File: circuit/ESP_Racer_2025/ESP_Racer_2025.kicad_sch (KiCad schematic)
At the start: 20 parts, among them IC1 XCL102D333CR-G, J1 Conn_LED_1, J2 Conn_LED_2, J3 Conn_Servo, U1 DRV8835DSST, U2 SFV12R-2STE1LF, U3 ESP32-C3-WROOM-02

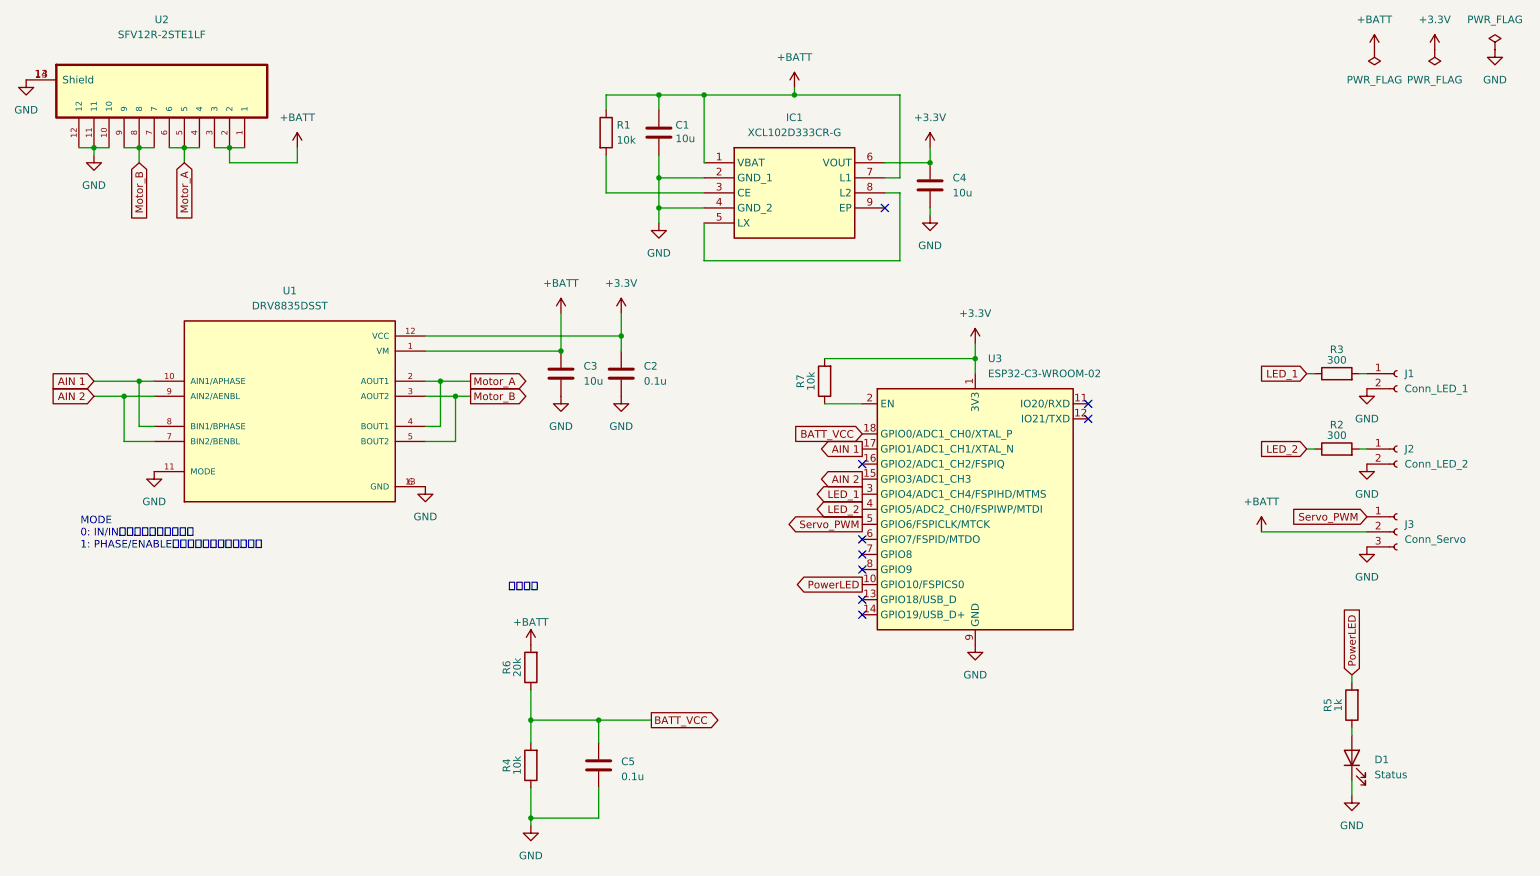
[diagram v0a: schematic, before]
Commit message: fix pcb
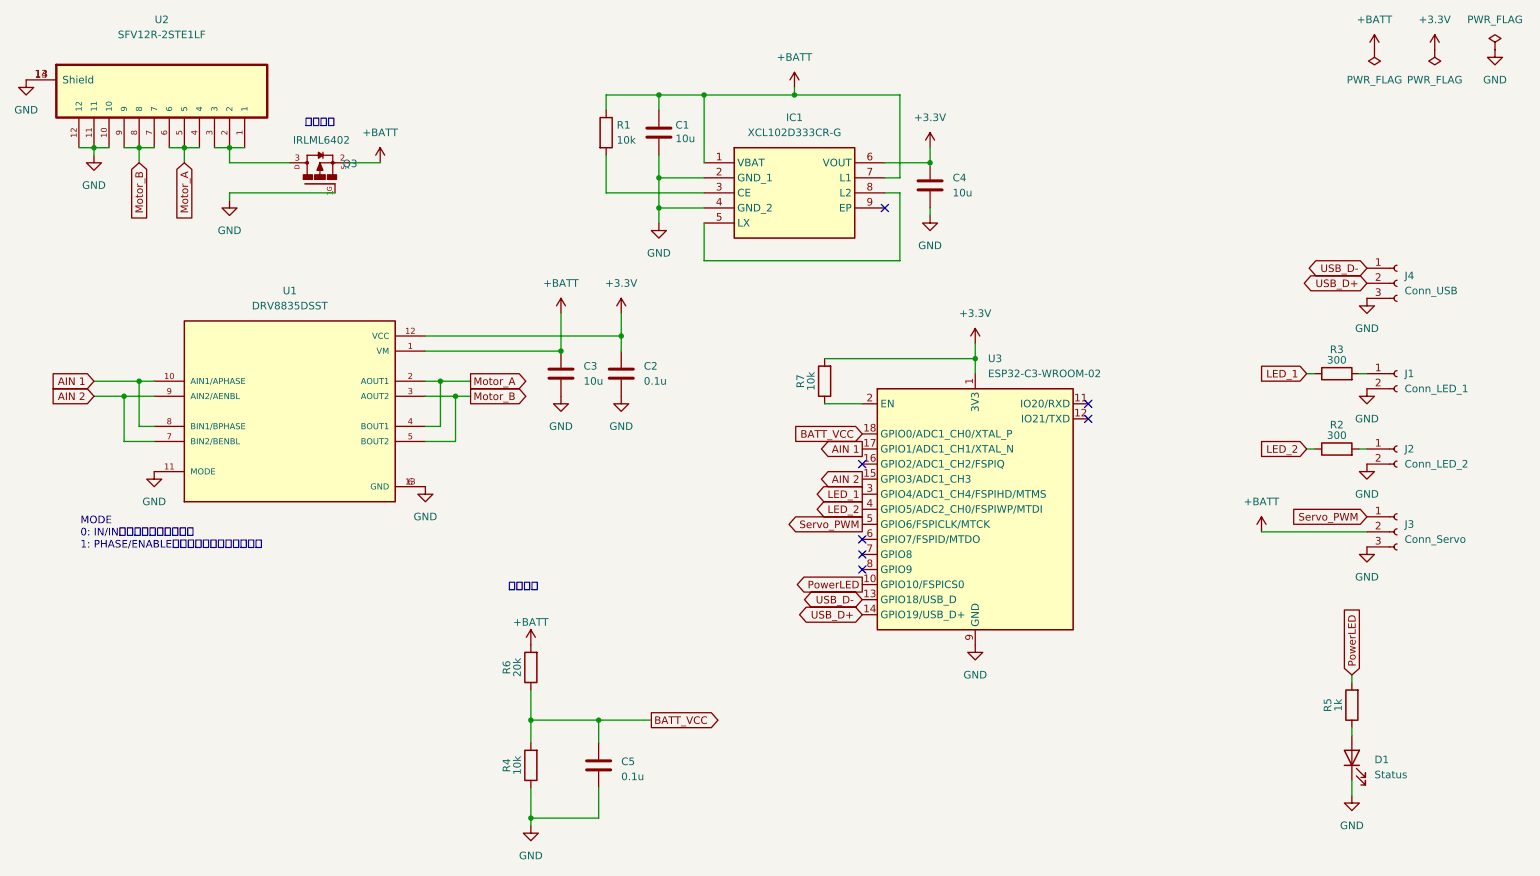
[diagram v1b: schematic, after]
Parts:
- added J4: Conn_USB, Original:Serial, symbol Connector:Conn_01x03_Socket
- added Q3: IRLML6402, IRLML6402:SOT23, symbol IRLML6402:IRLML6402
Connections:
- net +BATT: now also Q3.2; no longer U2.1, U2.2, U2.3
- net GND: now also J4.3 (Pin_3), Q3.1
- net USB_D-: now reaches U3.13 (GPIO18/USB_D)
- net USB_D-: now also J4.1 (Pin_1)
- net USB_D+: now reaches U3.14 (GPIO19/USB_D+)
- net USB_D+: now also J4.2 (Pin_2)
- new net: Q3.3, U2.1, U2.2, U2.3
- no-connect marks 9 -> 7
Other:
- note added: "逆接防止"

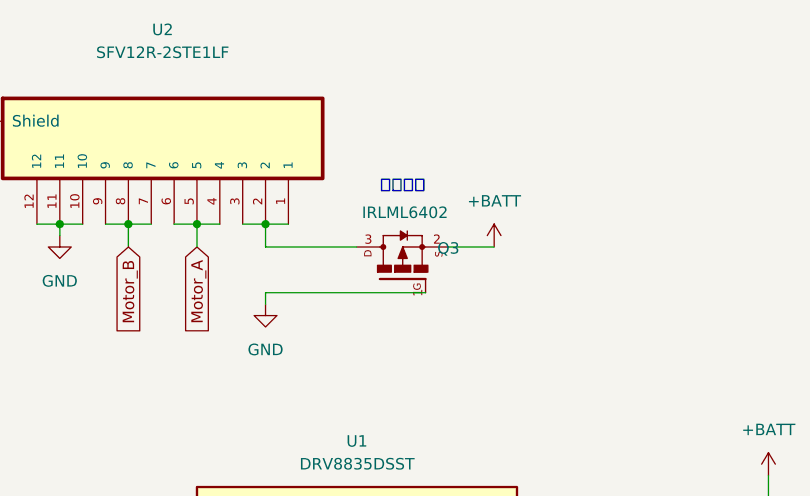
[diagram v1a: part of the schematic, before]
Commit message: pcb update
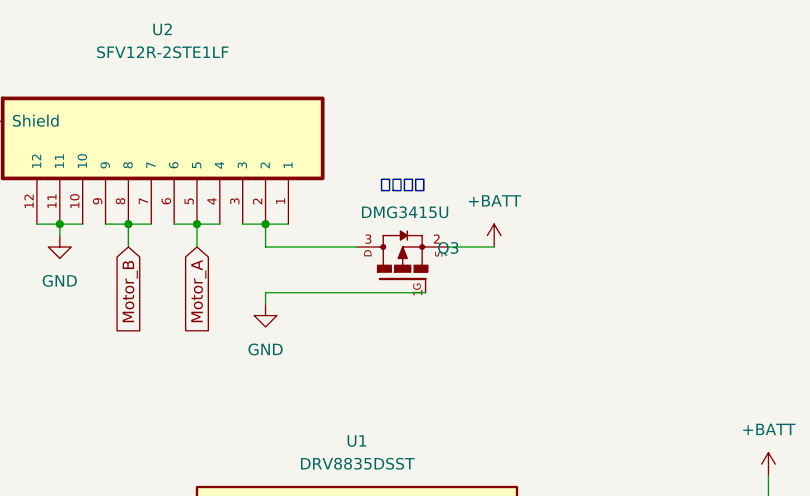
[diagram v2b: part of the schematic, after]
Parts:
- Q3: value IRLML6402 -> DMG3415U
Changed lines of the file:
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@@
 			)
 		)
-		(property "Value" "IRLML6402"
+		(property "Value" "DMG3415U"
 			(at 73.914 39.37 90)
 			(effects
